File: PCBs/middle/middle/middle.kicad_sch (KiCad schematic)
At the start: 28 parts, among them J15 Screw_Terminal_01x02, J16 Screw_Terminal_01x02, J17 Screw_Terminal_01x02, J18 Screw_Terminal_01x02, J19 Screw_Terminal_01x02, J2 Screw_Terminal_01x03, J21 Screw_Terminal_01x02, J3 Screw_Terminal_01x03, J4 Screw_Terminal_01x03, J5 Screw_Terminal_01x03, SW1 SW_Push, SW2 SW_Push, SW3 SW_Push, U1 DEV-16771, U2 4754, U3 RFM69HCW

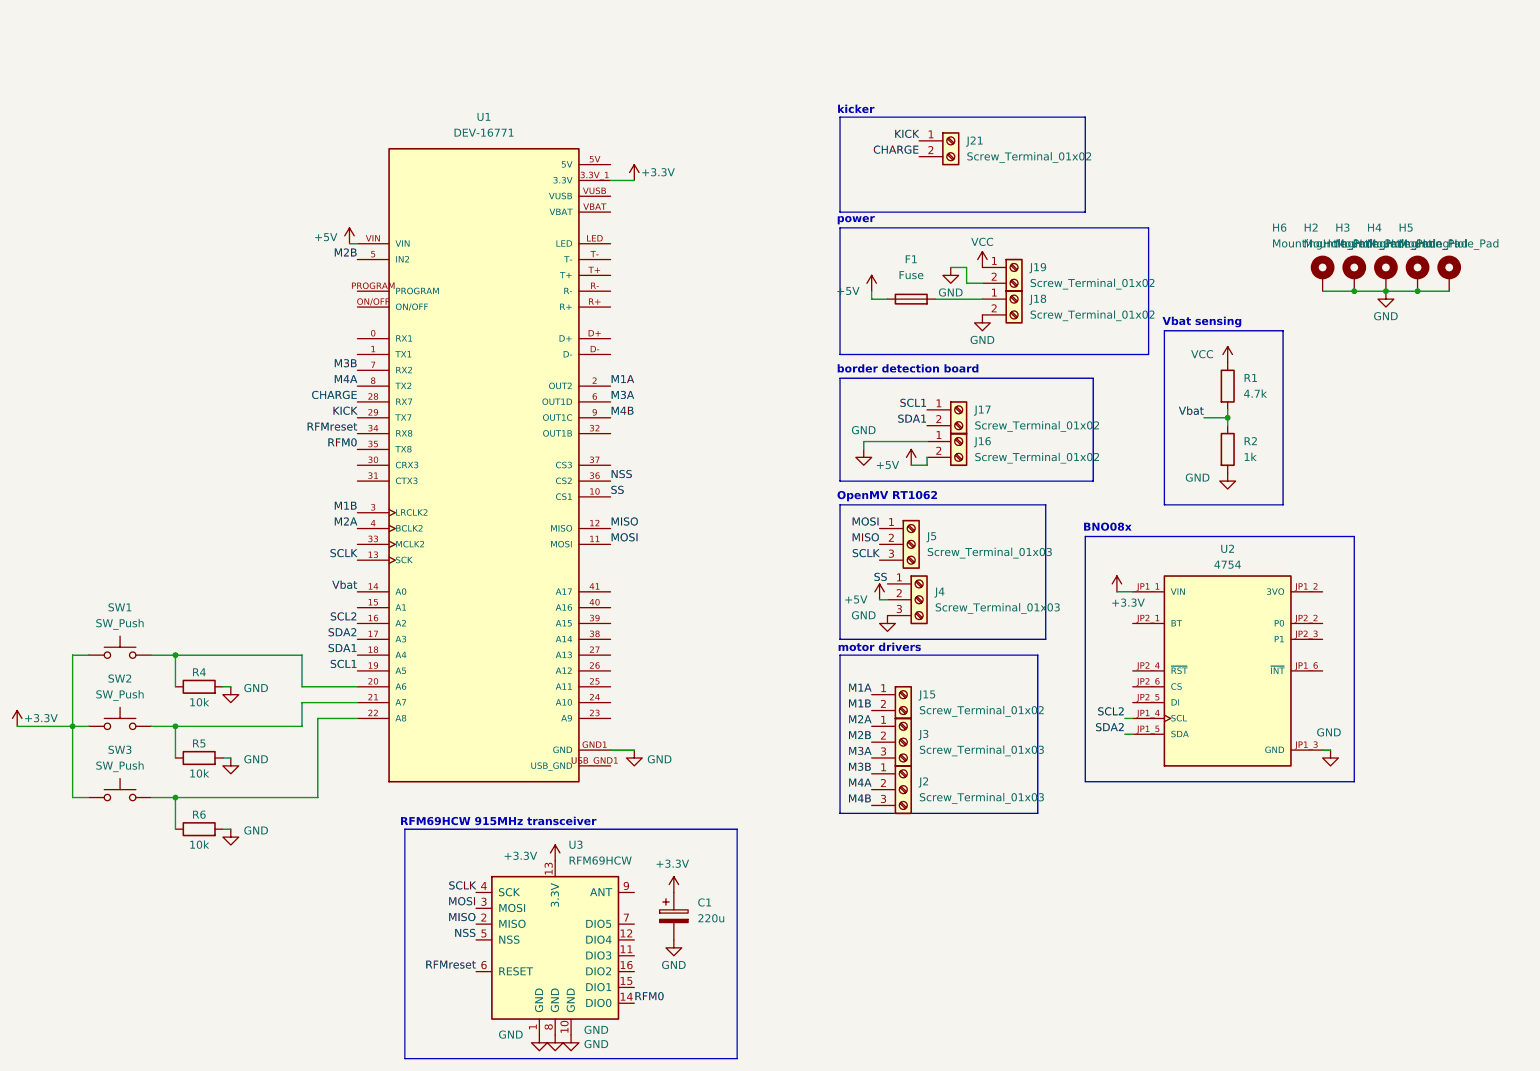
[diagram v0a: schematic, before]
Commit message: main update
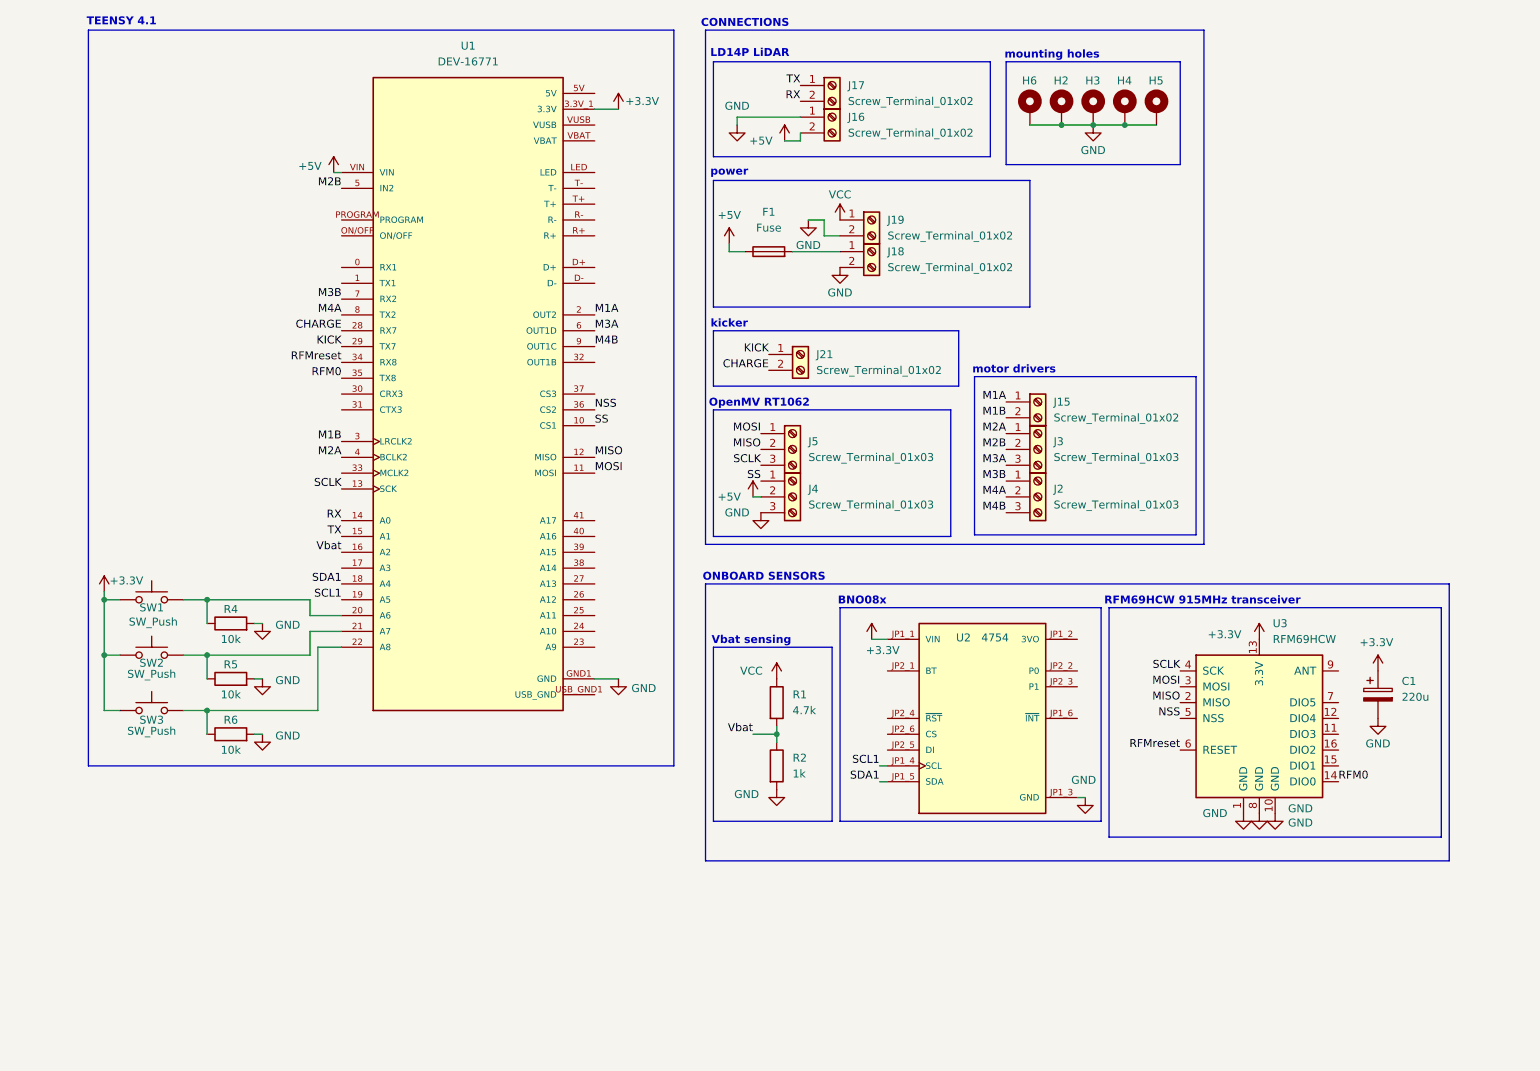
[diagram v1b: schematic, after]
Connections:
- net SCL1: now also U2.JP1_4 (SCL); no longer J17.1 (Pin_1)
- net SDA1: now also U2.JP1_5 (SDA); no longer J17.2 (Pin_2)
- net Vbat: now also U1.16 (A2); no longer U1.14 (A0)
- net TX: now reaches U1.15 (A1)
- net TX: now also J17.1 (Pin_1)
- removed net SCL2: U1.16 (A2), U2.JP1_4 (SCL)
- net SDA2: no longer names the net of U1.17 (A3)
- net SDA2: no longer U2.JP1_5 (SDA)
- new net RX: J17.2 (Pin_2), U1.14 (A0)
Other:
- note added: "CONNECTIONS"
- note added: "LD14P LiDAR"
- note added: "ONBOARD SENSORS"
- note added: "TEENSY 4.1"
- note added: "mounting holes"
- note removed: "border detection board"
- moved on the sheet: C1, F1, H2, H3, H4, H5, H6, J15, J16, J17, J18, J19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
